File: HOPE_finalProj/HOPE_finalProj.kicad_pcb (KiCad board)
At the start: 2 copper layers, 36 parts, among them M1 Mixer, SW1 SW_Push_DPDT, U1 LM386N-3_NOPB, U2 NE5534, U3 NE5534, U4 LM386N-3_NOPB, Y1 Crystal

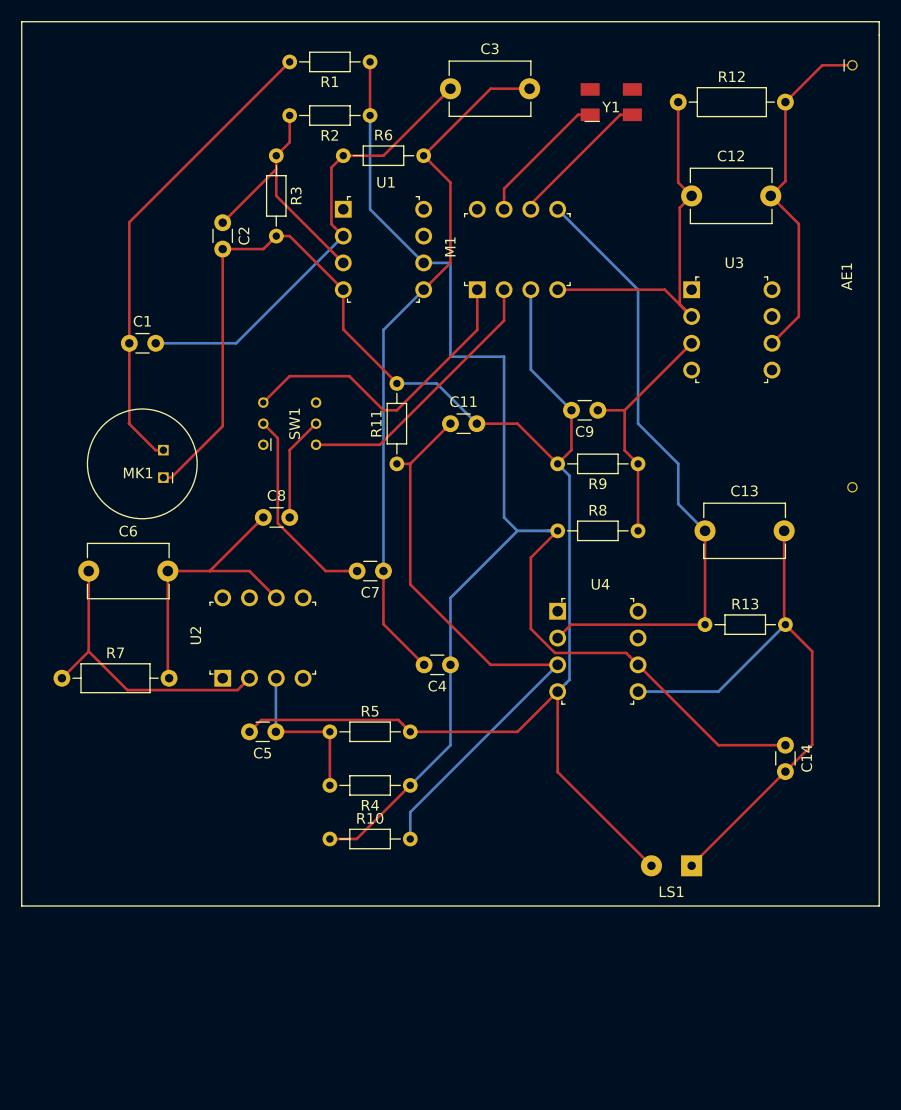
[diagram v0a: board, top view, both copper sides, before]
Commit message: Layout finished
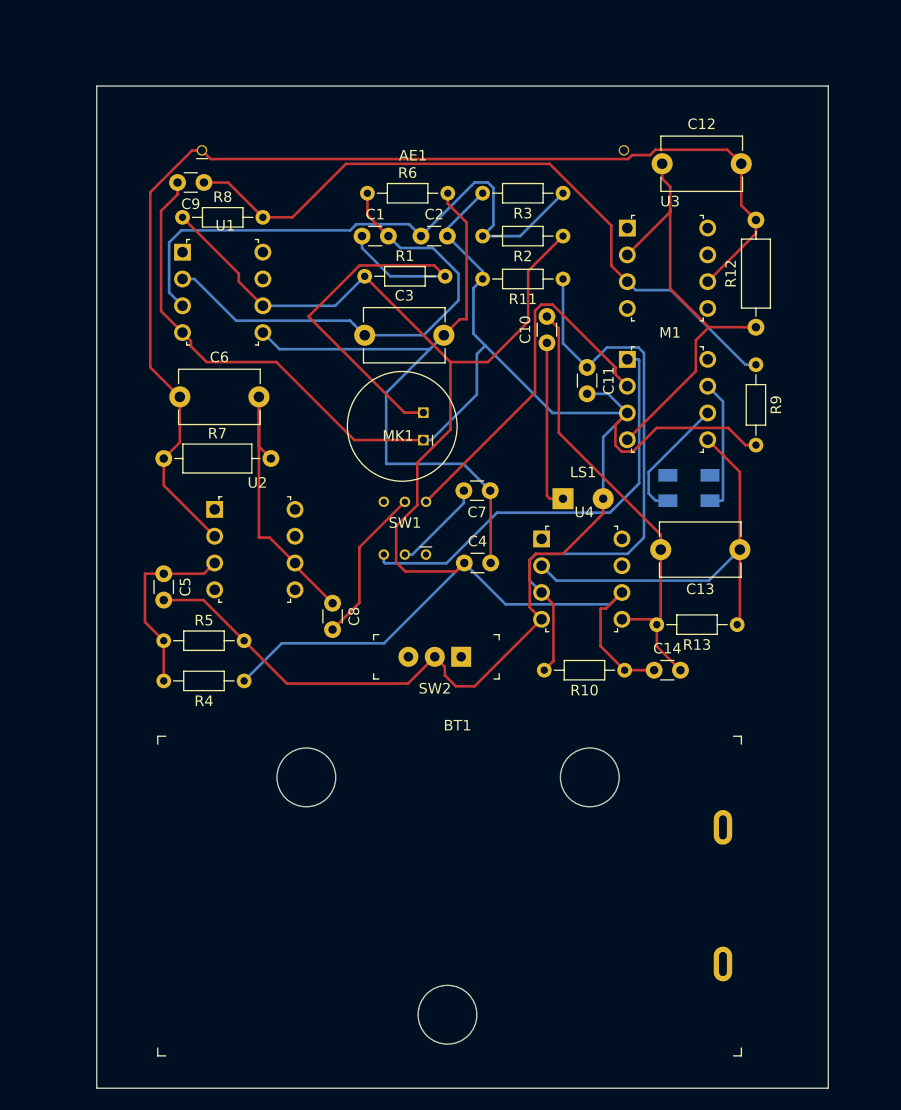
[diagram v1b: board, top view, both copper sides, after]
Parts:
- added BT1: Battery_Cell, digikey-footprints:Battery_Holder_9V_BC9VPC-ND, F.Cu at (150.4, 119.9)
- added C10: 1u, Capacitor_THT:C_Disc_D3.0mm_W1.6mm_P2.50mm, F.Cu at (146.3, 78.7)
- added SW2: SW_SPDT, digikey-footprints:Switch_Slide_11.6x4mm_EG1218, F.Cu at (138.2, 108.5)
- Y1: moved to B.Cu
- moved R8 46.3 mm to (111.8, 66.8)
- moved AE1 43.3 mm to (133.6, 60.5), turned to 0 degrees
- moved C9 43.1 mm to (113.8, 63.5)
- moved Y1 37.3 mm to (159.8, 92.5), turned to 180 degrees
- moved LS1 36.9 mm to (147.8, 93.5), turned to 0 degrees
- moved R10 32.2 mm to (153.7, 109.7), turned to 180 degrees
- moved R3 27.4 mm to (147.8, 64.5), turned to 180 degrees
- moved MK1 24.9 mm to (132.6, 86.6)
- moved C3 24.7 mm to (129.0, 78.0)
- moved C1 24.3 mm to (128.8, 68.6)
- moved R11 23.6 mm to (147.8, 72.6), turned to 180 degrees
- moved R7 23.0 mm to (110.0, 89.7)
- moved R12 22.6 mm to (166.1, 77.2), turned to 90 degrees
- moved R2 21.6 mm to (147.8, 68.6)
- moved R1 20.3 mm to (129.0, 72.4), turned to 0 degrees
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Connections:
- AE1 pad 1: Net-(AE1-Pad1) -> /ANT
- C12 pad 2: Net-(AE1-Pad1) -> /ANT
- C13 pad 2: Net-(C13-Pad2) -> Net-(C10-Pad2)
- C14 pad 2: Net-(C13-Pad2) -> Net-(C10-Pad2)
- C6 pad 1: Net-(C6-Pad1) -> /ANT
- LS1 pad 1: Net-(C13-Pad2) -> Net-(C10-Pad1)
- R12 pad 2: Net-(AE1-Pad1) -> /ANT
- R13 pad 2: Net-(C13-Pad2) -> Net-(C10-Pad2)
- R7 pad 1: Net-(C6-Pad1) -> /ANT
- U2 pad 2: Net-(C6-Pad1) -> /ANT
- U3 pad 6: Net-(AE1-Pad1) -> /ANT
- U4 pad 5: Net-(C13-Pad2) -> Net-(C10-Pad2)
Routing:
- net /ANT: track 0.00 -> 112.4 mm
- net Net-(C13-Pad2): track 54.2 -> 0.00 mm
- net Net-(C10-Pad2): track 0.00 -> 42.6 mm
- net Net-(C9-Pad1): track 23.5 -> 65.9 mm
- net Net-(AE1-Pad1): track 33.4 -> 0.00 mm
- net Net-(C2-Pad1): track 24.3 -> 55.1 mm
- net Net-(C6-Pad1): track 28.4 -> 0.00 mm
- net GND: track 161.0 -> 182.1 mm
- net Net-(C13-Pad1): track 59.7 -> 39.5 mm
- net Net-(C10-Pad1): track 0.00 -> 16.1 mm
- net Net-(M1-Pad1): track 29.6 -> 40.9 mm
- net Net-(C7-Pad2): track 19.4 -> 8.78 mm
- net Net-(M1-Pad2): track 25.6 -> 35.0 mm
- net Net-(C12-Pad1): track 35.5 -> 41.9 mm
- net Net-(C8-Pad2): track 9.93 -> 15.0 mm
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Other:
- board outline added: 69.3 x 95 mm
